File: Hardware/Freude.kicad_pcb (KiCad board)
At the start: 4 copper layers, 110.2 x 37.2 mm, 43 parts, among them J1 Conn_01x06_Female, J10 Conn_01x06_Female, J11 Conn_01x05_Male, J12 Conn_01x05_Female, J2 Conn_01x05_Female, J3 Conn_01x06_Female, J4 Conn_01x04_Female, J5 Conn_01x04_Female, J6 Conn_01x04_Male, J7 Conn_01x03_Female, J8 Conn_01x06_Male, J9 Conn_01x06_Female, SW1 B3FS-1015P`, U1 IQS572, U2 STM32L432KBUx, U3 TLV713185PDBV, X1 Custom_Touchpad, Y1 Crystal_GND24

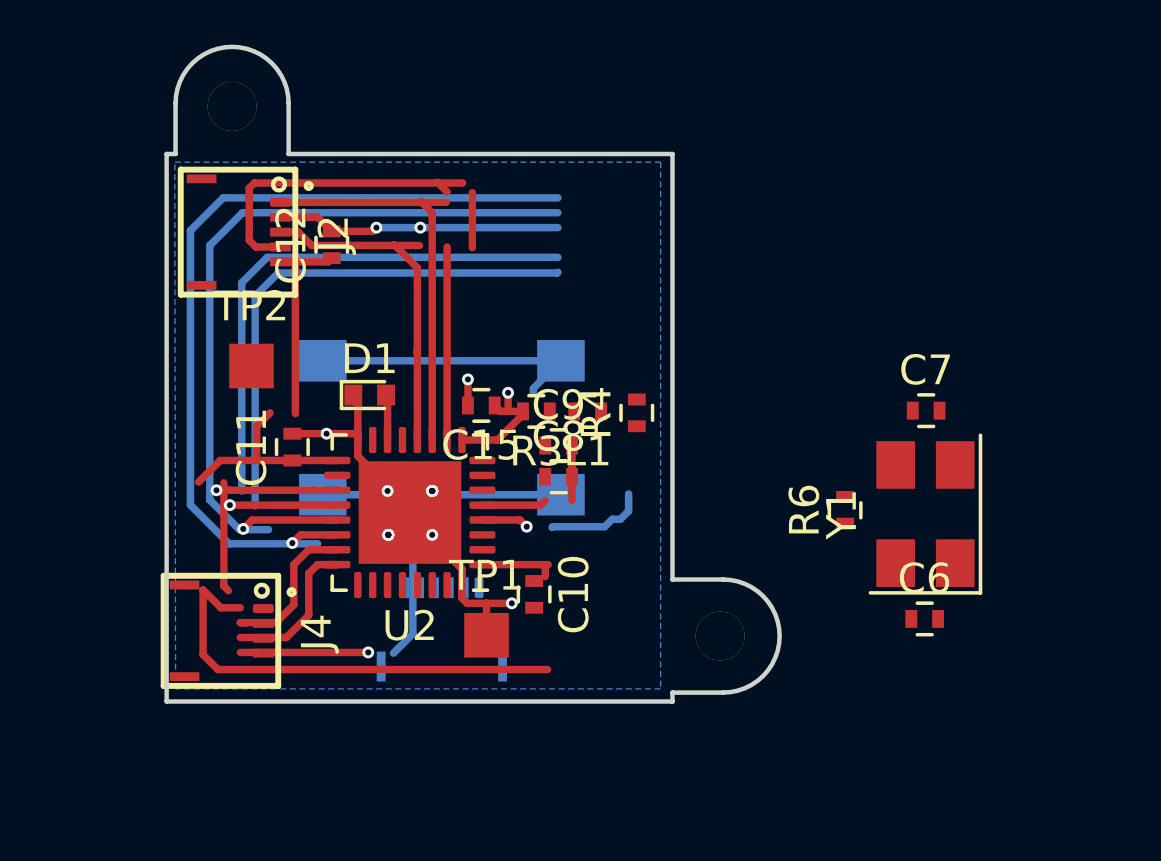
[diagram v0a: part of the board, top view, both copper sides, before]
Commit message: rerouted, tidied
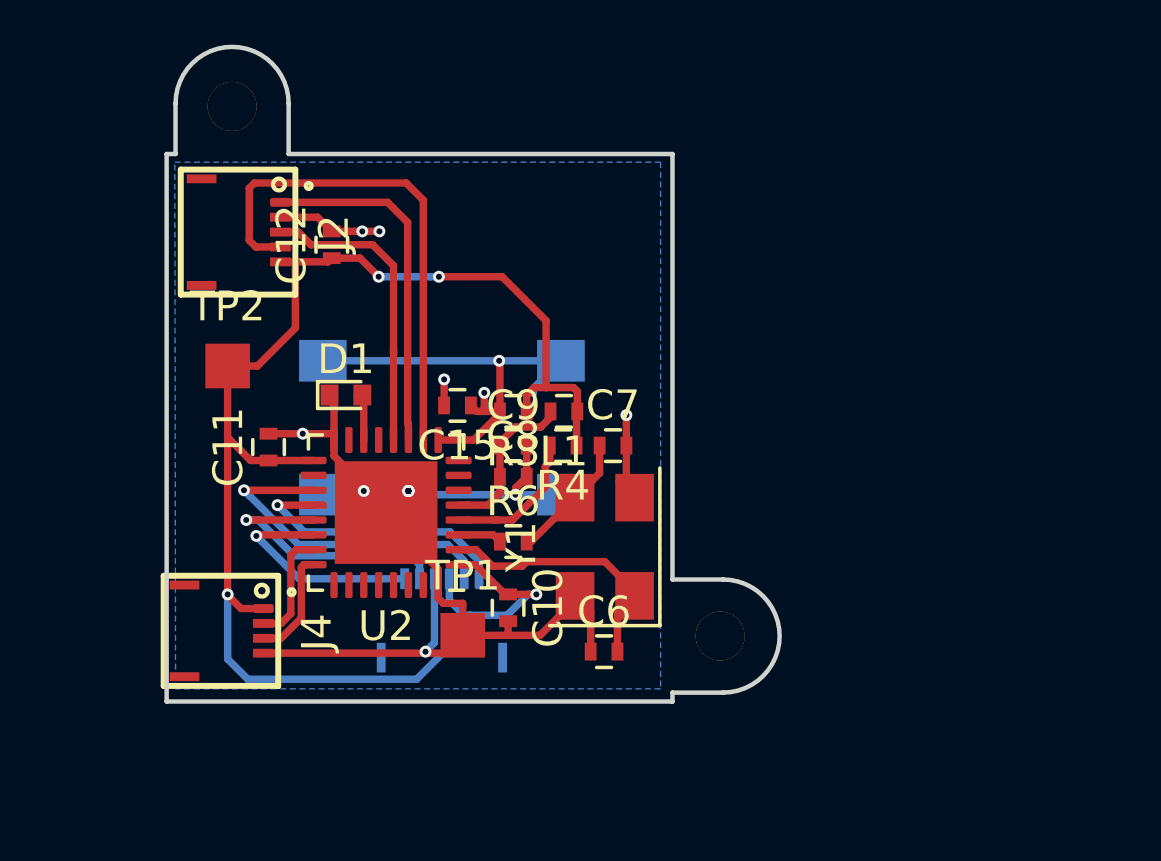
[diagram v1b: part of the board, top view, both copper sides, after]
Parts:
- moved R6 11.2 mm to (203.1, 83.7), turned to 0 degrees
- moved Y1 10.8 mm to (206.2, 83.8)
- moved C6 10.8 mm to (206.2, 87.3)
- moved C7 10.6 mm to (206.5, 80.4)
- moved R4 2.71 mm to (204.8, 80.4), turned to 180 degrees
- moved C8 1.53 mm to (203.1, 81.5)
- moved C9 1.53 mm to (203.1, 80.4)
- moved C10 0.98 mm to (202.9, 85.9)
- moved C15 0.80 mm to (201.2, 79.1)
- moved D1 0.80 mm to (197.5, 78.7)
- moved L1 0.80 mm to (204.8, 79.3)
- moved U2 0.80 mm to (198.8, 82.7)
- moved C11 0.80 mm to (194.9, 80.5)
- moved TP1 0.80 mm to (201.4, 86.8)
- moved TP2 0.80 mm to (193.5, 77.8)
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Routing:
- net /AZO_UNK: track 28.5 -> 7.52 mm
- net /RDY_UC: track 26.4 -> 9.18 mm
- net +3V3: track 35.4 -> 52.6 mm, vias 0 -> 4
- net /SDA_UC: track 21.2 -> 9.42 mm
- net /SCL_UC: track 22.0 -> 11.3 mm
- net Net-(C6-Pad2): track 0.00 -> 8.88 mm
- net Net-(C7-Pad1): track 0.00 -> 5.14 mm
- net Net-(C8-Pad1): track 2.17 -> 5.51 mm
- net GND: track 44.2 -> 47.2 mm, vias 16 -> 13
- net /DAC2_OUT1: track 13.7 -> 11.9 mm
- net /DAC1_OUT2: track 18.9 -> 17.1 mm
- net /SWCLK: track 5.46 -> 3.71 mm
- net /Switch_In: track 13.6 -> 15.4 mm, vias 1 -> 2
- net /Switch_Out: track 11.9 -> 10.3 mm
- net Net-(R6-Pad1): track 0.00 -> 1.48 mm
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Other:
- net class Default: clearance 0.018 -> 0.1
- rule trace_clearance: 0.018 -> 0.1
